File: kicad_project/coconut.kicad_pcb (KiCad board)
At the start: 2 copper layers, 212.6 x 79.2 mm, 88 parts

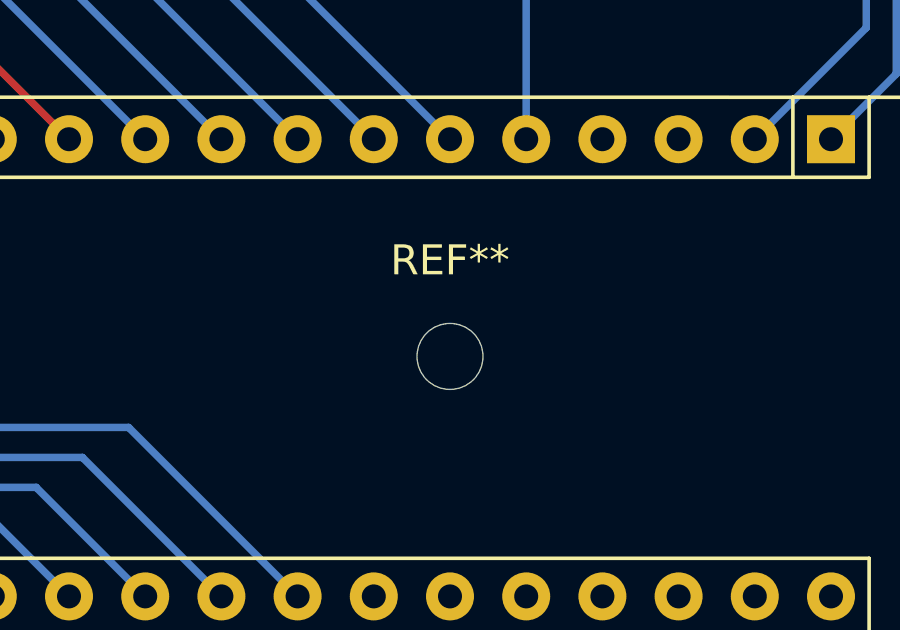
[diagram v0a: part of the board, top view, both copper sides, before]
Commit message: fix holes
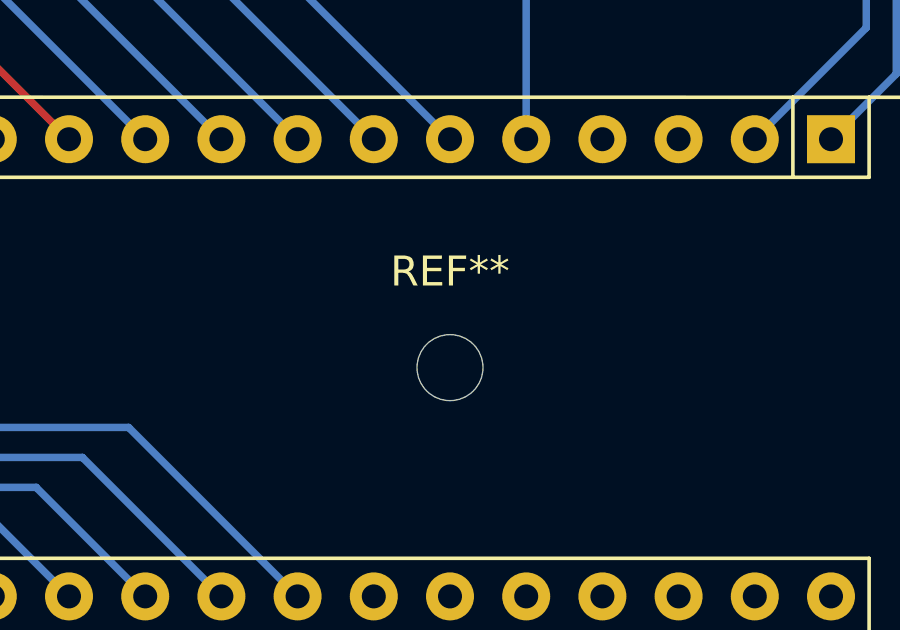
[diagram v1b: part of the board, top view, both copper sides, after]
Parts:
- moved REF** 0.37 mm to (195.2, 68.5)
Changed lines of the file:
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@@
   )
   (footprint "MountingHole:MountingHole_2.2mm_M2" (layer "F.Cu")
-    (at 195.175 68.177)
+    (at 195.175 68.55)
     (descr "Mounting Hole 2.2mm, no annular, M2")
     (tags "mounting hole 2.2mm no annular m2")
